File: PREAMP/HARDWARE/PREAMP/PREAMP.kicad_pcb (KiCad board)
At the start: 2 copper layers, 1 part, among them U1 TL074

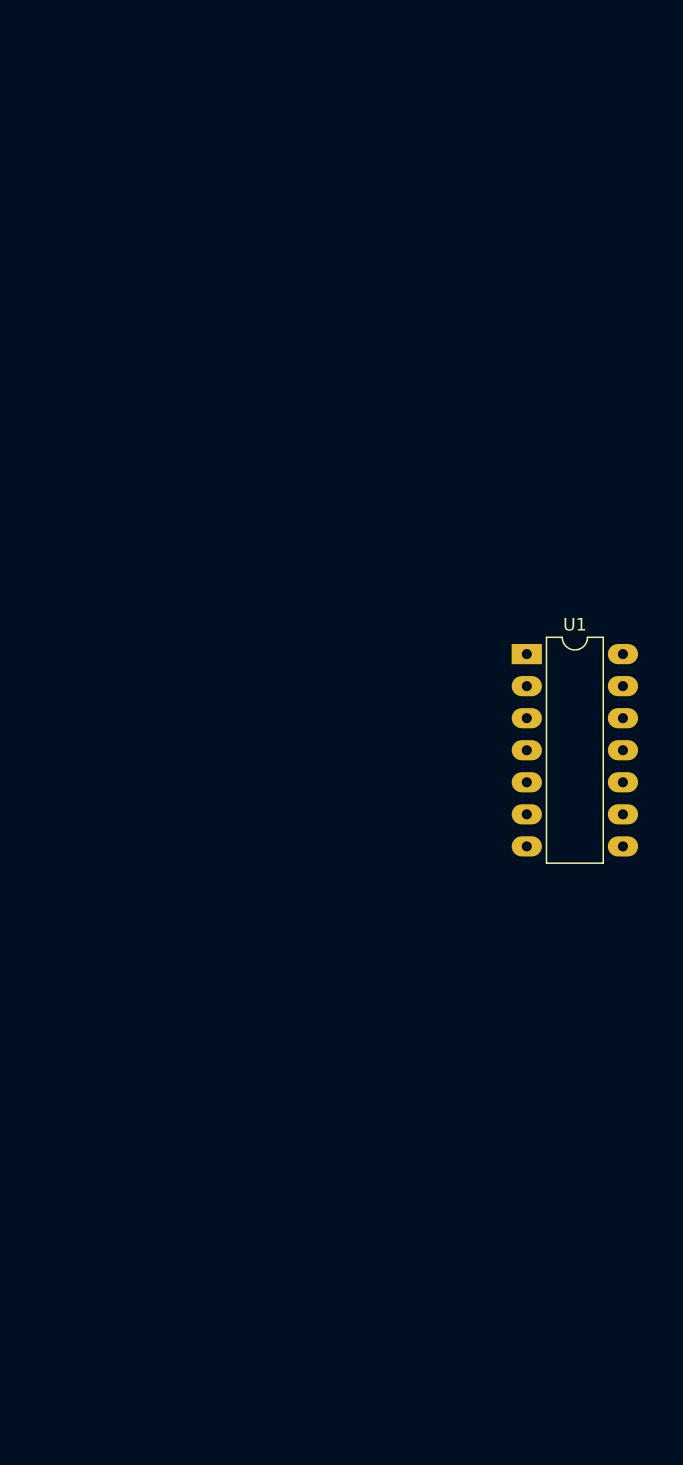
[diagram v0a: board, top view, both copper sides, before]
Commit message: Initial Board Layout
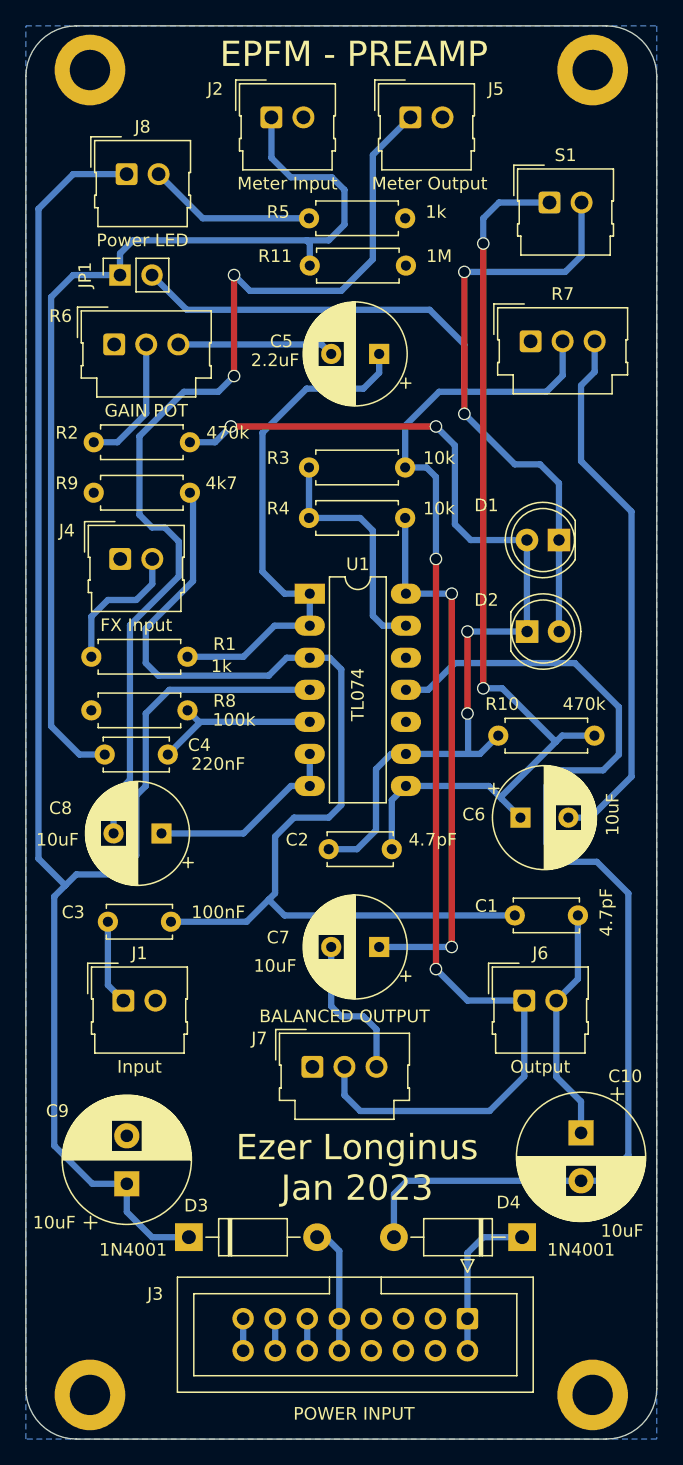
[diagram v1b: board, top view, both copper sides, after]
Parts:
- added C1: 4.7pF, Capacitor_THT:C_Disc_D5.0mm_W2.5mm_P5.00mm, F.Cu at (143.8, 110.5)
- added C10: 10uF, Capacitor_THT:CP_Radial_D10.0mm_P3.80mm, F.Cu at (144.0, 127.7)
- added C2: 4.7pF, Capacitor_THT:C_Disc_D5.0mm_W2.5mm_P5.00mm, F.Cu at (129.0, 105.2)
- added C3: 100nF, Capacitor_THT:C_Disc_D5.0mm_W2.5mm_P5.00mm, F.Cu at (106.5, 111.0)
- added C4: 220nF, Capacitor_THT:C_Disc_D5.0mm_W2.5mm_P5.00mm, F.Cu at (111.2, 97.8)
- added C5: 2.2uF, Capacitor_THT:CP_Radial_D8.0mm_P3.80mm, F.Cu at (128.0, 66.0)
- added C6: 10uF, Capacitor_THT:CP_Radial_D8.0mm_P3.80mm, F.Cu at (139.2, 102.8)
- added C7: 10uF, Capacitor_THT:CP_Radial_D8.0mm_P3.80mm, F.Cu at (128.0, 113.0)
- added C8: 10uF, Capacitor_THT:CP_Radial_D8.0mm_P3.80mm, F.Cu at (110.8, 104.0)
- added C9: 10uF, Capacitor_THT:CP_Radial_D10.0mm_P3.80mm, F.Cu at (108.0, 131.8)
- added D1: LED, LED_THT:LED_D5.0mm, F.Cu at (142.2, 80.8)
- added D2: LED, LED_THT:LED_D5.0mm, F.Cu at (139.7, 88.0)
- added D3: 1N4001, Diode_THT:D_DO-41_SOD81_P10.16mm_Horizontal, F.Cu at (112.9, 136.0)
- added D4: 1N4001, Diode_THT:D_DO-41_SOD81_P10.16mm_Horizontal, F.Cu at (139.3, 136.0)
- added H1: MountingHole, MountingHole:MountingHole_3.2mm_M3_DIN965_Pad, F.Cu at (105.1, 43.5)
- added H2: MountingHole, MountingHole:MountingHole_3.2mm_M3_DIN965_Pad, F.Cu at (144.9, 43.5)
- added H3: MountingHole, MountingHole:MountingHole_3.2mm_M3_DIN965_Pad, F.Cu at (105.1, 148.5)
- added H4: MountingHole, MountingHole:MountingHole_3.2mm_M3_DIN965_Pad, F.Cu at (144.9, 148.5)
- added J1: Input, Connector_Molex:Molex_SL_171971-0002_1x02_P2.54mm_Vertical, F.Cu at (107.7, 117.2)
- added J2: Meter Input, Connector_Molex:Molex_SL_171971-0002_1x02_P2.54mm_Vertical, F.Cu at (119.5, 47.2)
- added J3: POWER INPUT, Connector_IDC:IDC-Header_2x08_P2.54mm_Vertical, F.Cu at (135.0, 142.5)
- added J4: FX Input, Connector_Molex:Molex_SL_171971-0002_1x02_P2.54mm_Vertical, F.Cu at (107.5, 82.2)
- added J5: Meter Output, Connector_Molex:Molex_SL_171971-0002_1x02_P2.54mm_Vertical, F.Cu at (130.5, 47.2)
- added J6: Output, Connector_Molex:Molex_SL_171971-0002_1x02_P2.54mm_Vertical, F.Cu at (139.5, 117.2)
- added J7: BALANCED OUTPUT, Connector_Molex:Molex_SL_171971-0003_1x03_P2.54mm_Vertical, F.Cu at (122.7, 122.5)
- added J8: Power LED, Connector_Molex:Molex_SL_171971-0002_1x02_P2.54mm_Vertical, F.Cu at (108.0, 51.8)
- added JP1: Jumper_2_Open, Connector_PinSocket_2.54mm:PinSocket_1x02_P2.54mm_Vertical, F.Cu at (107.5, 59.8)
- added R1: 1k, Resistor_THT:R_Axial_DIN0207_L6.3mm_D2.5mm_P7.62mm_Horizontal, F.Cu at (105.2, 90.0)
- added R10: 470k, Resistor_THT:R_Axial_DIN0207_L6.3mm_D2.5mm_P7.62mm_Horizontal, F.Cu at (137.4, 96.2)
- added R11: 1M, Resistor_THT:R_Axial_DIN0207_L6.3mm_D2.5mm_P7.62mm_Horizontal, F.Cu at (122.5, 59.0)
- added R2: 4k7, Resistor_THT:R_Axial_DIN0207_L6.3mm_D2.5mm_P7.62mm_Horizontal, F.Cu at (105.4, 73.0)
- added R3: 10k, Resistor_THT:R_Axial_DIN0207_L6.3mm_D2.5mm_P7.62mm_Horizontal, F.Cu at (122.4, 75.0)
- added R4: 10k, Resistor_THT:R_Axial_DIN0207_L6.3mm_D2.5mm_P7.62mm_Horizontal, F.Cu at (122.4, 79.0)
- added R5: 1k, Resistor_THT:R_Axial_DIN0207_L6.3mm_D2.5mm_P7.62mm_Horizontal, F.Cu at (130.1, 55.2)
- added R6: GAIN POT, Connector_Molex:Molex_SL_171971-0003_1x03_P2.54mm_Vertical, F.Cu at (107.0, 65.2)
- added R7: MASTER, Connector_Molex:Molex_SL_171971-0003_1x03_P2.54mm_Vertical, F.Cu at (140.0, 65.0)
- added R8: 100k, Resistor_THT:R_Axial_DIN0207_L6.3mm_D2.5mm_P7.62mm_Horizontal, F.Cu at (112.8, 94.2)
- added R9: 470k, Resistor_THT:R_Axial_DIN0207_L6.3mm_D2.5mm_P7.62mm_Horizontal, F.Cu at (113.0, 77.0)
- added S1: CLEAN/DIRTY, Connector_Molex:Molex_SL_171971-0002_1x02_P2.54mm_Vertical, F.Cu at (141.5, 54.0)
- moved U1 17.9 mm to (122.5, 85.0)
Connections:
- U1 pad 1: unconnected-(U1-Pad1) -> Net-(C5-Pad1)
- U1 pad 10: unconnected-(U1-Pad10) -> Earth
- U1 pad 11: unconnected-(U1-Pad11) -> Net-(C10-Pad2)
- U1 pad 12: unconnected-(U1-Pad12) -> Earth
- U1 pad 13: unconnected-(U1-Pad13) -> Net-(R3-Pad1)
- U1 pad 14: unconnected-(U1-Pad14) -> Net-(C7-Pad1)
- U1 pad 2: unconnected-(U1-Pad2) -> Net-(C5-Pad1)
- U1 pad 3: unconnected-(U1-Pad3) -> Net-(C1-Pad2)
- U1 pad 4: unconnected-(U1-Pad4) -> Net-(C9-Pad1)
- U1 pad 5: unconnected-(U1-Pad5) -> Net-(C4-Pad1)
- U1 pad 6: unconnected-(U1-Pad6) -> Net-(C8-Pad1)
- U1 pad 7: unconnected-(U1-Pad7) -> Net-(C8-Pad1)
- U1 pad 8: unconnected-(U1-Pad8) -> Net-(C2-Pad1)
- U1 pad 9: unconnected-(U1-Pad9) -> Net-(C2-Pad2)
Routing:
- net Net-(C9-Pad1): track 0.00 -> 130.5 mm
- net Net-(R3-Pad2): track 0.00 -> 124.9 mm, vias 0 -> 2
- net Net-(C10-Pad2): track 0.00 -> 86.4 mm
- net Net-(C1-Pad2): track 0.00 -> 82.8 mm
- net Net-(C4-Pad2): track 0.00 -> 80.7 mm
- net Net-(C8-Pad2): track 0.00 -> 78.0 mm, vias 0 -> 2
- net Net-(C2-Pad2): track 0.00 -> 76.3 mm, vias 0 -> 4
- net Net-(C2-Pad1): track 0.00 -> 75.7 mm, vias 0 -> 2
- net Net-(D1-Pad1): track 0.00 -> 46.8 mm, vias 0 -> 2
- net Net-(C7-Pad1): track 0.00 -> 43.4 mm, vias 0 -> 2
- net Net-(C6-Pad2): track 0.00 -> 43.0 mm
- net Net-(C5-Pad1): track 0.00 -> 41.4 mm
- net Net-(R3-Pad1): track 0.00 -> 19.2 mm
- net Earth: track 0.00 -> 18.3 mm
- net Net-(C8-Pad1): track 0.00 -> 15.8 mm
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- added copper zone on B.Cu, net Earth
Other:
- board outline added: 50 x 112 mm
- board text added: "EPFM - PREAMP"
- board text added: "Ezer Longinus Jan 2023"
